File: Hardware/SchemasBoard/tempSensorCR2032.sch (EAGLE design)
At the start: 11 parts, among them IC1 DS1820, T2 BC846

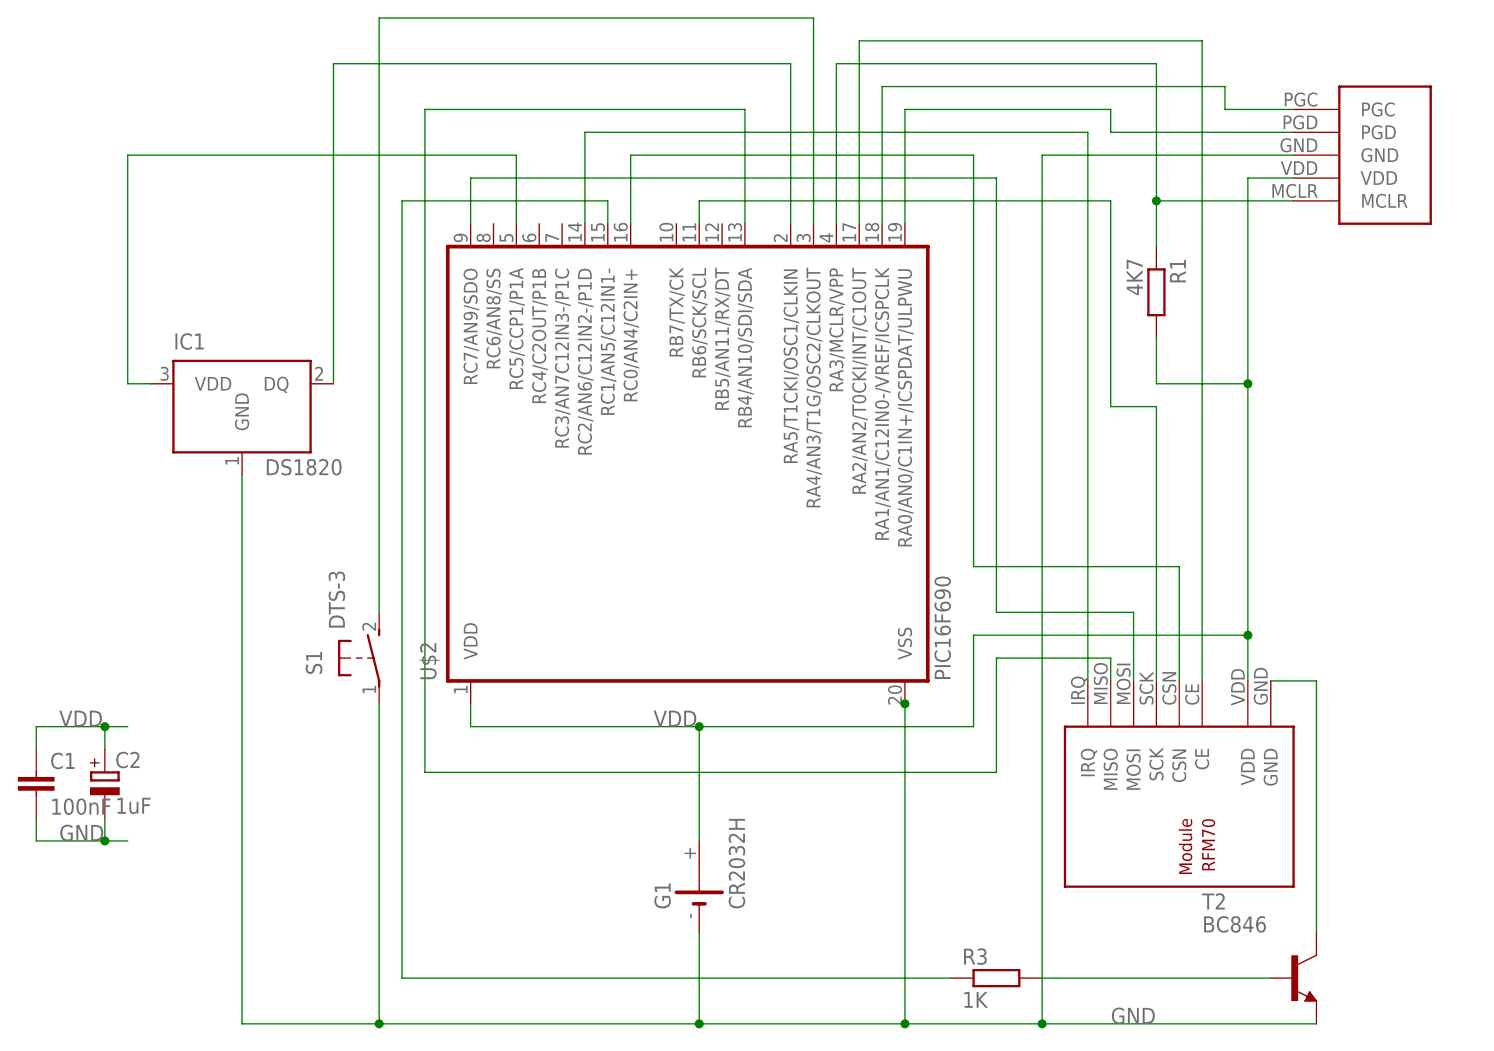
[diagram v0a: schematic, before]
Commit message: hf
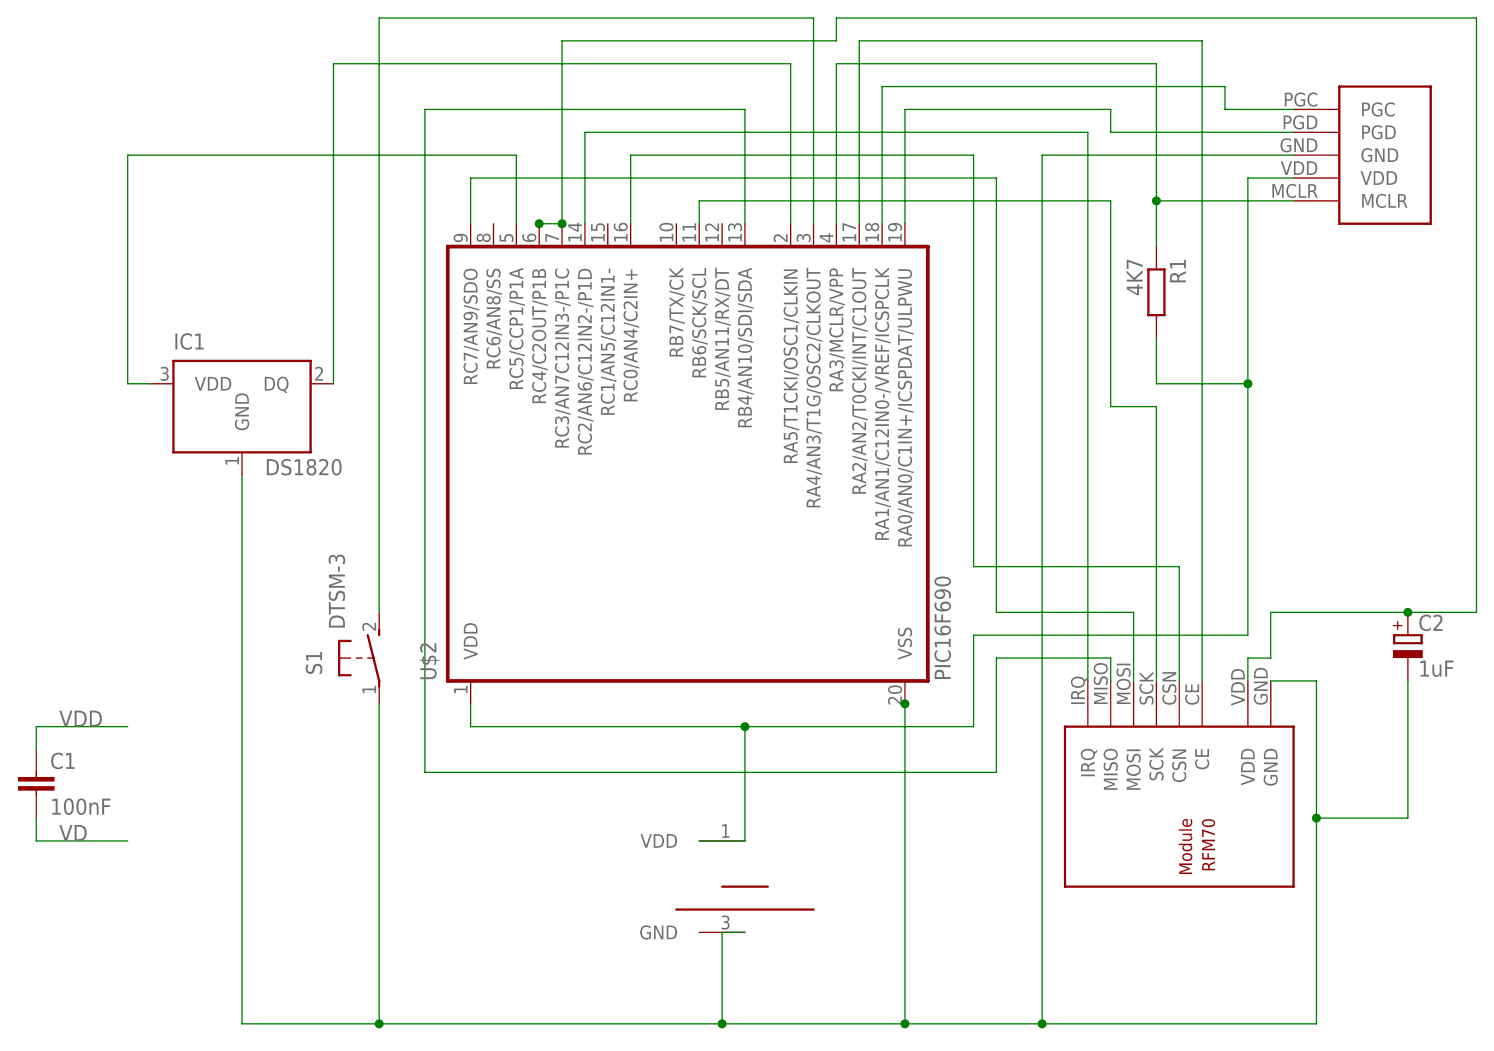
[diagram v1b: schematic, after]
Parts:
- removed G1: CR2032H, battery:CR2032H
- removed R3: 1K, resistor:R-EU_R1206W
- removed T2: BC846, transistor:BC846
- added U$4: CR2032, rfm70:CR2032
- S1: value DTS-3 -> DTSM-3; device switch-tact:DTS-3 -> switch-tact:DTSM-3
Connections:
- removed net GND: C1.2, C2.-, G1.-, IC1.GND, S1.1, T2.E, U$2.VSS, U$3.GND
- removed net N$13: T2.C, U$1.GND
- removed net N$14: R3.2, T2.B
- removed net N$15: R3.1, U$2.RC1/AN5/C12IN1-
- new net N$4: C2.+, U$1.VDD, U$2.RC3/AN7C12IN3-/P1C, U$2.RC4/C2OUT/P1B
- new net N$5: R1.2, U$2.VDD, U$3.VDD, U$4.VDD
- new net VD: C1.2, C2.-, IC1.GND, S1.1, U$1.GND, U$2.VSS, U$3.GND, U$4.GND
- net VDD: no longer C2.+, G1.+, R1.2, U$1.VDD, U$2.VDD, U$3.VDD
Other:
- moved on the sheet: C2
